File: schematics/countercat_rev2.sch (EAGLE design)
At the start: 57 parts, among them IC1 74LS595N, Q2 2N3904, Q3 IRF520, Q4 IRF520, U4 ATMEGA328P_PDIP, U6 RELAYPTH3, Y1 16MHz

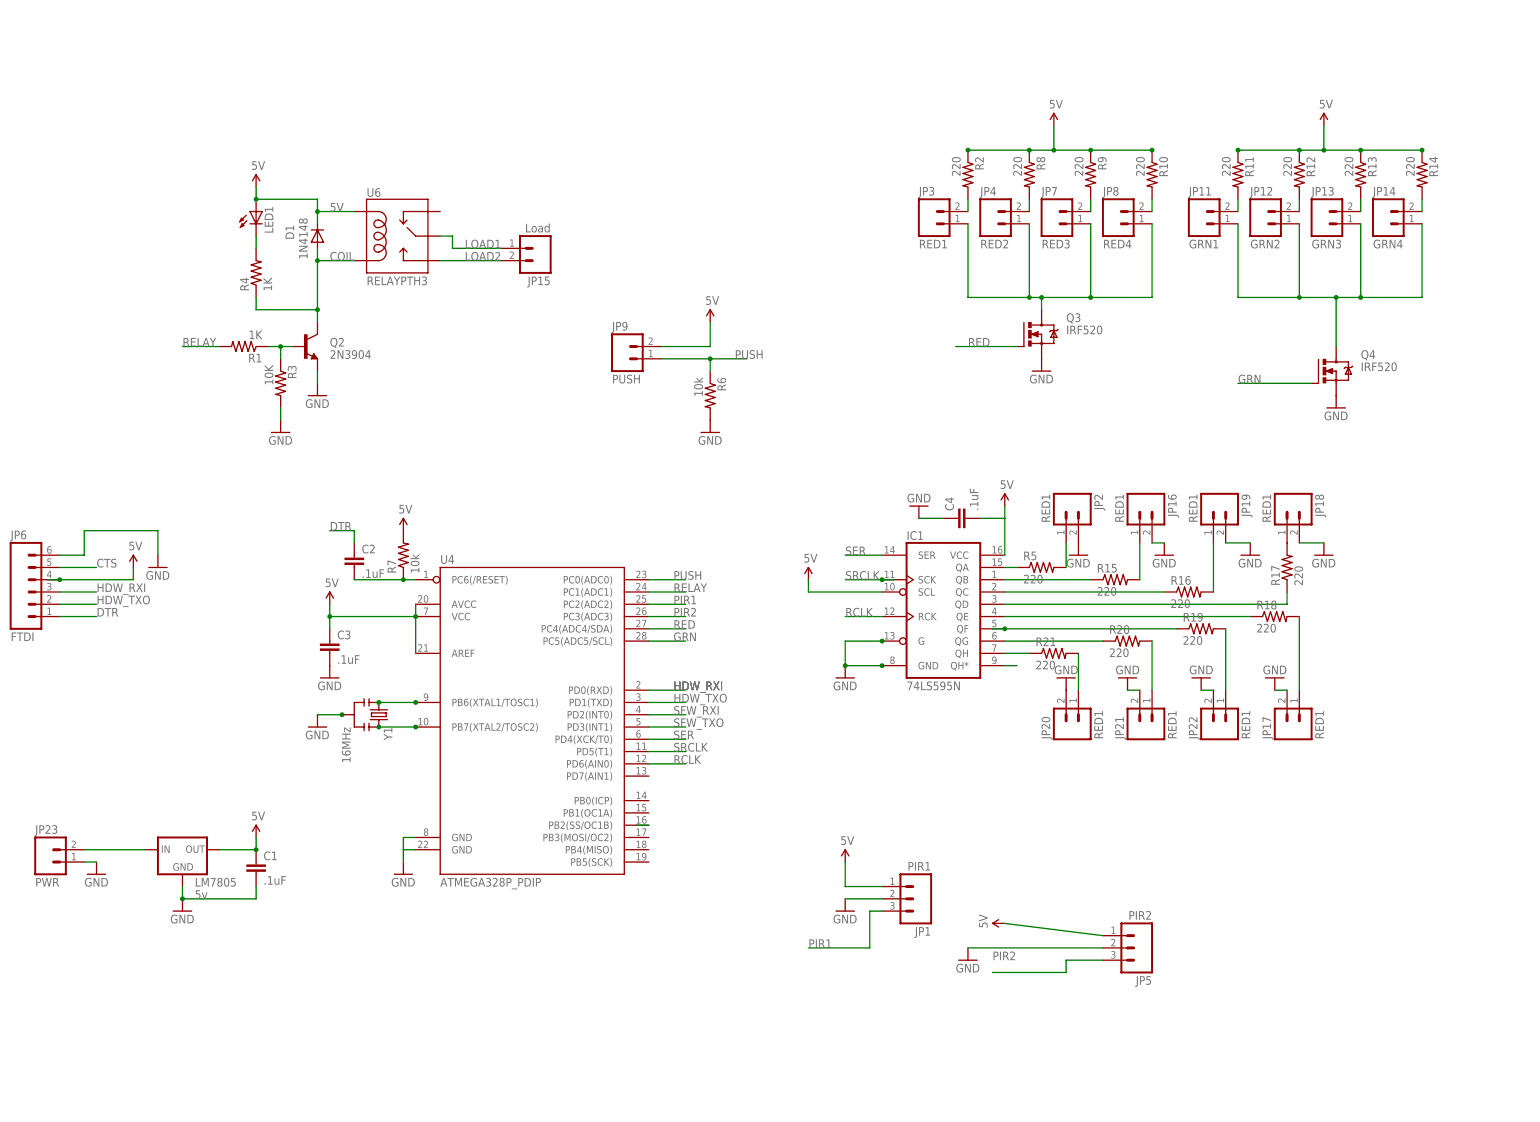
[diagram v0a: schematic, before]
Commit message: Updated board and schematic
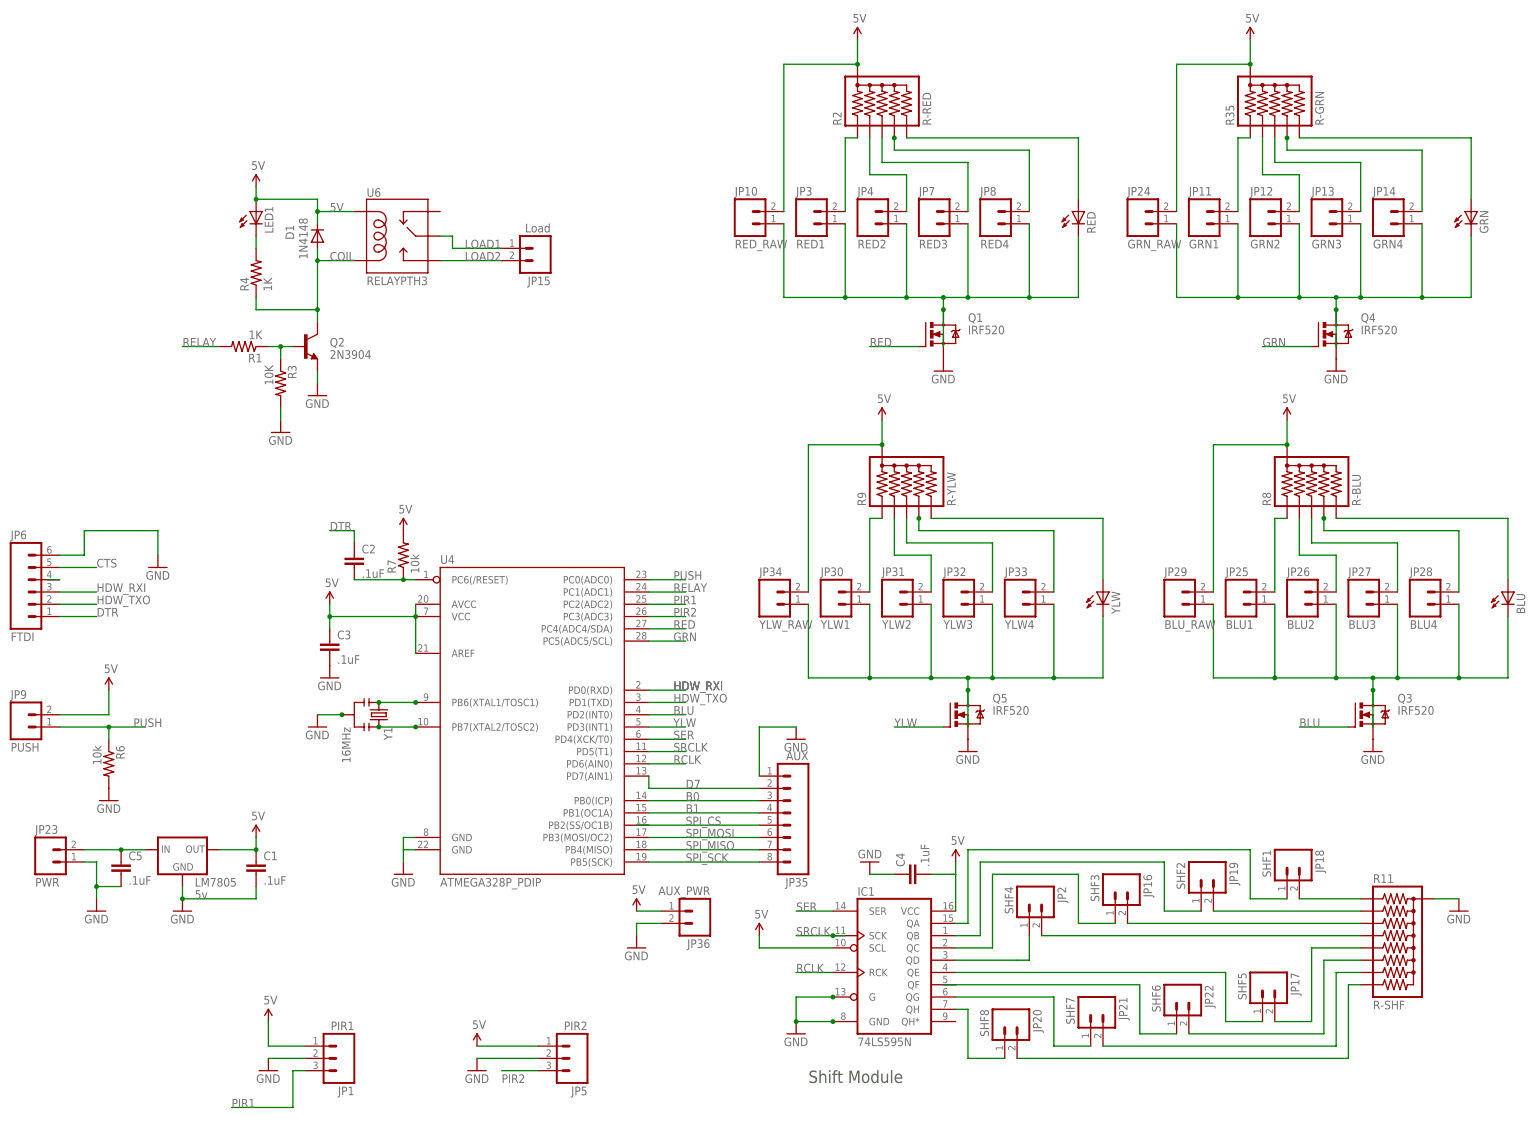
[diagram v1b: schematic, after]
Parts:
- removed R10, R12, R13, R14, R15, R16, R17, R18, R19, R20, R21, R5: 220, SparkFun-Resistors:RESISTORPTH-1/4W
- added BLU, GRN, RED, YLW: (no value), SparkFun-LED:LED3MM
- added C5: .1uF, SparkFun-Capacitors:CAPPTH2
- added JP10: RED_RAW, SparkFun:M02POLAR
- added JP24: GRN_RAW, SparkFun:M02POLAR
- added JP25: BLU1, SparkFun:M02POLAR
- added JP26: BLU2, SparkFun:M02POLAR
- added JP27: BLU3, SparkFun:M02POLAR
- added JP28: BLU4, SparkFun:M02POLAR
- added JP29: BLU_RAW, SparkFun:M02POLAR
- added JP30: YLW1, SparkFun:M02POLAR
- added JP31: YLW2, SparkFun:M02POLAR
- added JP32: YLW3, SparkFun:M02POLAR
- added JP33: YLW4, SparkFun:M02POLAR
- added JP34: YLW_RAW, SparkFun:M02POLAR
- added JP35: AUX, SparkFun-Connectors:M08LOCK
- added JP36: AUX_PWR, SparkFun:M02POLAR
- added Q1, Q5: IRF520, transistor-power:IRF520
- added R35: R-GRN, SparkFun-Resistors:RPACK-BUSSED-5-SIP-PTH-5
- JP16: value RED1 -> SHF3
- JP17: value RED1 -> SHF5
- JP18: value RED1 -> SHF1
- JP19: value RED1 -> SHF2
- JP2: value RED1 -> SHF4
- JP20: value RED1 -> SHF8
- JP21: value RED1 -> SHF7
- JP22: value RED1 -> SHF6
- R11: value 220 -> R-SHF; device SparkFun-Resistors:RESISTORPTH-1/4W -> SparkFun-Resistors:RPACK-BUSSED-8-SIP-PTH-8
- R2: value 220 -> R-RED; device SparkFun-Resistors:RESISTORPTH-1/4W -> SparkFun-Resistors:RPACK-BUSSED-5-SIP-PTH-5
- R8: value 220 -> R-BLU; device SparkFun-Resistors:RESISTORPTH-1/4W -> SparkFun-Resistors:RPACK-BUSSED-5-SIP-PTH-5
- R9: value 220 -> R-YLW; device SparkFun-Resistors:RESISTORPTH-1/4W -> SparkFun-Resistors:RPACK-BUSSED-5-SIP-PTH-5
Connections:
- removed net N$22 (its old number): JP8.2, R10.2
- removed net SFW_RXI: U4.PD2(INT0)
- removed net SFW_TXO: U4.PD3(INT1)
- new net B0: JP35.3, U4.PB0(ICP)
- new net B1: JP35.4, U4.PB1(OC1A)
- new net BLU: Q3.G, U4.PD2(INT0)
- new net D7: JP35.2, U4.PD7(AIN1)
- new net N$12: JP4.2, R2.3
- new net N$18: JP7.2, R2.4
- new net N$34: BLU.C, JP25.1, JP26.1, JP27.1, JP28.1, JP29.1, Q3.D
- new net N$35: JP26.2, R8.3
- new net N$36: JP27.2, R8.4
- new net N$37: JP28.2, R8.5
- new net N$38: BLU.A, R8.6
- new net N$39: JP25.2, R8.2
- new net N$40: JP30.1, JP31.1, JP32.1, JP33.1, JP34.1, Q5.D, YLW.C
- new net N$41: JP31.2, R9.3
- new net N$42: JP32.2, R9.4
- new net N$43: JP33.2, R9.5
- new net N$44: R9.6, YLW.A
- new net N$45: GRN.A, R35.6
- new net N$46: JP30.2, R9.2
- new net SPI_MISO: JP35.7, U4.PB4(MISO)
- new net SPI_MOSI: JP35.6, U4.PB3(MOSI/OC2)
- new net SPI_SCK: JP35.8, U4.PB5(SCK)
- new net YLW: Q5.G, U4.PD3(INT1)
- net 5V: now also JP10.2, JP24.2, JP29.2, JP34.2, JP36.1, R35.1; no longer JP6.4, R10.1, R11.1, R12.1, R13.1, R14.1
- net GND: now also C5.2, JP35.1, JP36.2, Q1.S, Q5.S, R11.1; no longer JP16.2, JP17.2, JP18.2, JP19.2, JP2.2, JP20.2, JP21.2, JP22.2
- net N$1: now also IC1.QE, JP17.1; no longer IC1.QH*
- net N$10: now also JP18.2, R11.2; no longer JP2.1, R5.2
- net N$11: now also JP19.2, R11.3; no longer JP16.1, R15.2
- net N$13: now also R35.3; no longer R12.2
- net N$14: now also JP16.2, R11.4; no longer JP19.1, R16.2
- net N$15: now also R35.4; no longer R13.2
- net N$16: now also R35.5; no longer R14.2
- net N$17: now also JP2.2, R11.5; no longer JP18.1, R17.2
- net N$19: now also JP8.2, R2.5; no longer JP4.2, R8.2
- net N$2: now also JP10.1, Q1.D, RED.C; no longer Q3.D
- net N$20: now also JP17.2, R11.6; no longer JP17.1, R18.2
- net N$21: now also R2.6, RED.A; no longer JP7.2, R9.2
- net N$23: now also JP22.2, R11.7; no longer JP22.1, R19.2
- net N$24: now also JP21.2, R11.8; no longer JP21.1, R20.2
- net N$25: now also JP20.2, R11.9; no longer JP20.1, R21.2
- net N$26: now also JP18.1; no longer R5.1
- net N$27: now also JP19.1; no longer R15.1
- net N$28: now also JP16.1; no longer R16.1
- net N$29: now also JP2.1; no longer R17.1
- net N$30: now also IC1.QG, JP21.1; no longer IC1.QE, R18.1
- net N$31: now also JP22.1; no longer R19.1
- net N$32: now also IC1.QH, JP20.1; no longer IC1.QG, R20.1
- net N$33: now also JP6.4; no longer IC1.QH, R21.1
- net N$4: now also GRN.C, JP24.1, Q4.D
- net N$5: now also R35.2; no longer R11.2
- net RED: now also Q1.G; no longer Q3.G
- net SPI_CS: now also JP35.5
- net VB: now also C5.1
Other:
- note added: "Shift Module"
- moved on the sheet: C4, IC1, JP1, JP16, JP17, JP18, JP19, JP2, JP20, JP21, JP22, JP3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
